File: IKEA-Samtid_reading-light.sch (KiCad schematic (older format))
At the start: 20 parts, among them IC1 ATTINY25-S, P1 CONN_2, U1 PT4115-SOT89-5

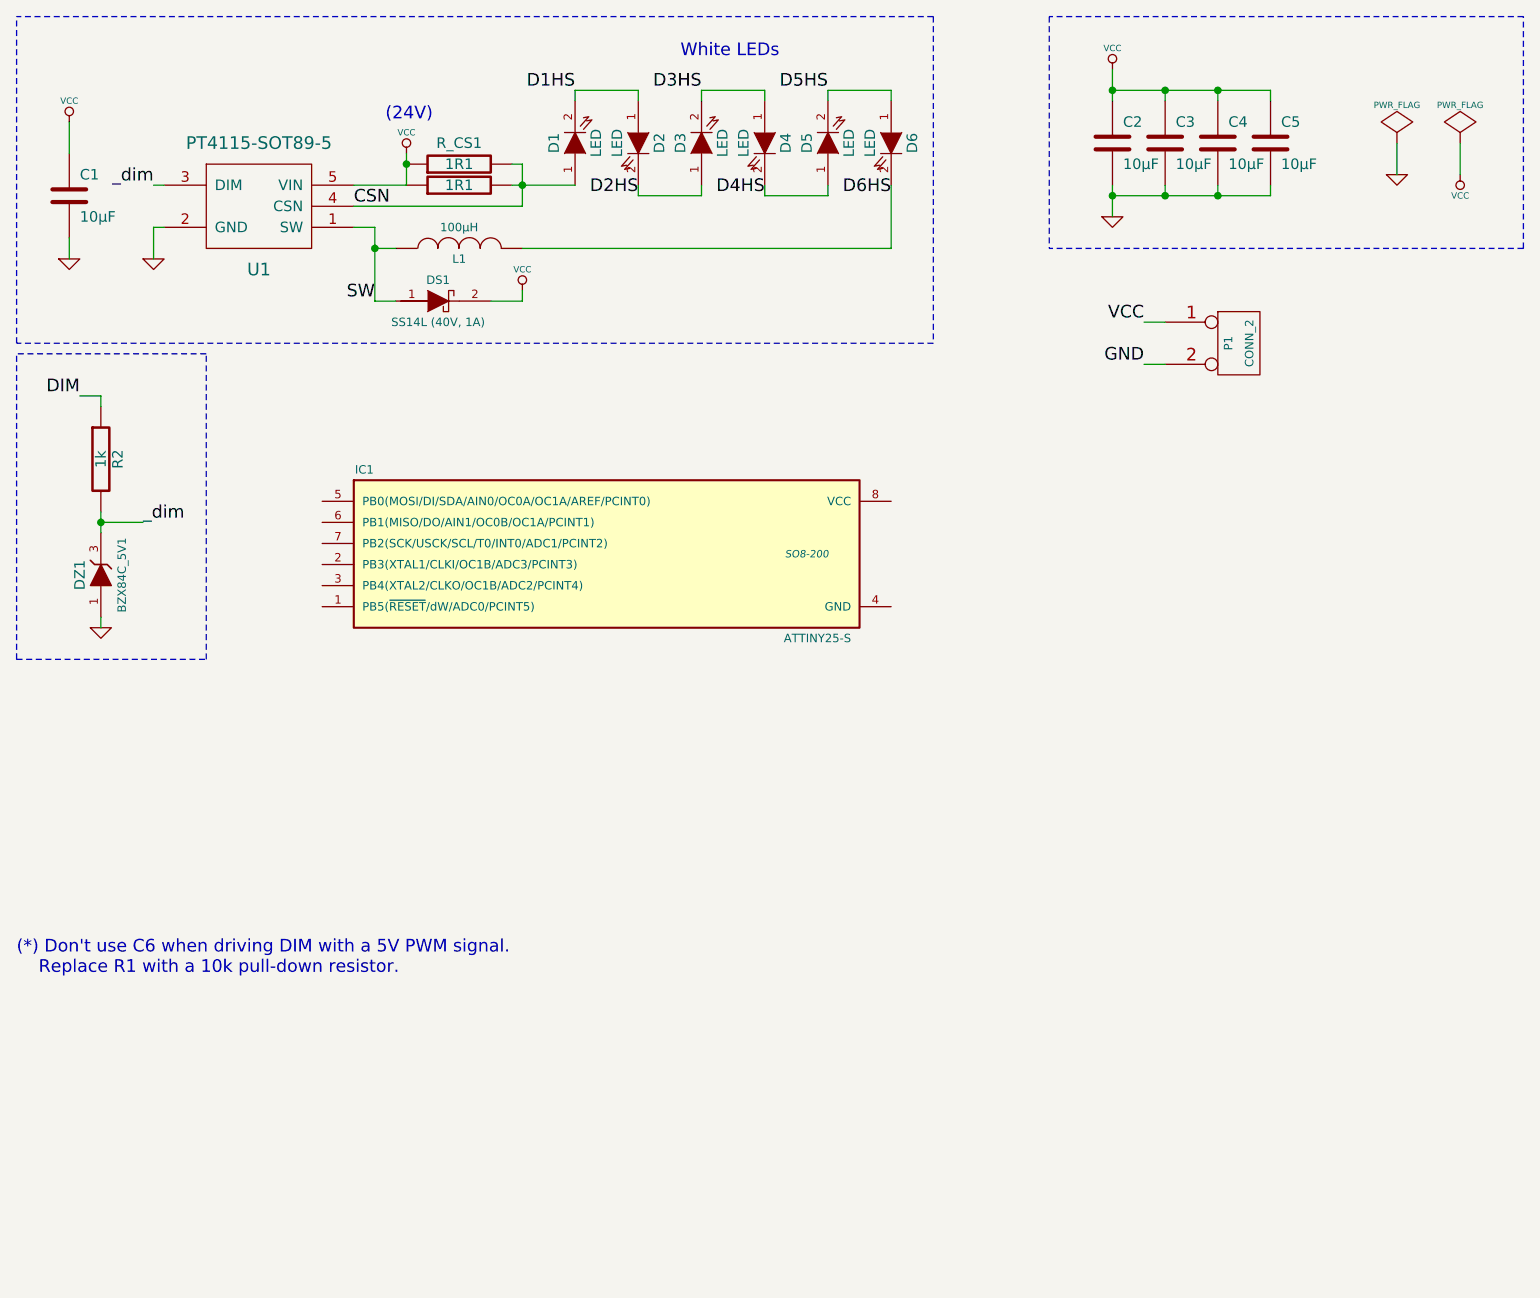
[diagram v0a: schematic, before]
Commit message: Shoving parts around.
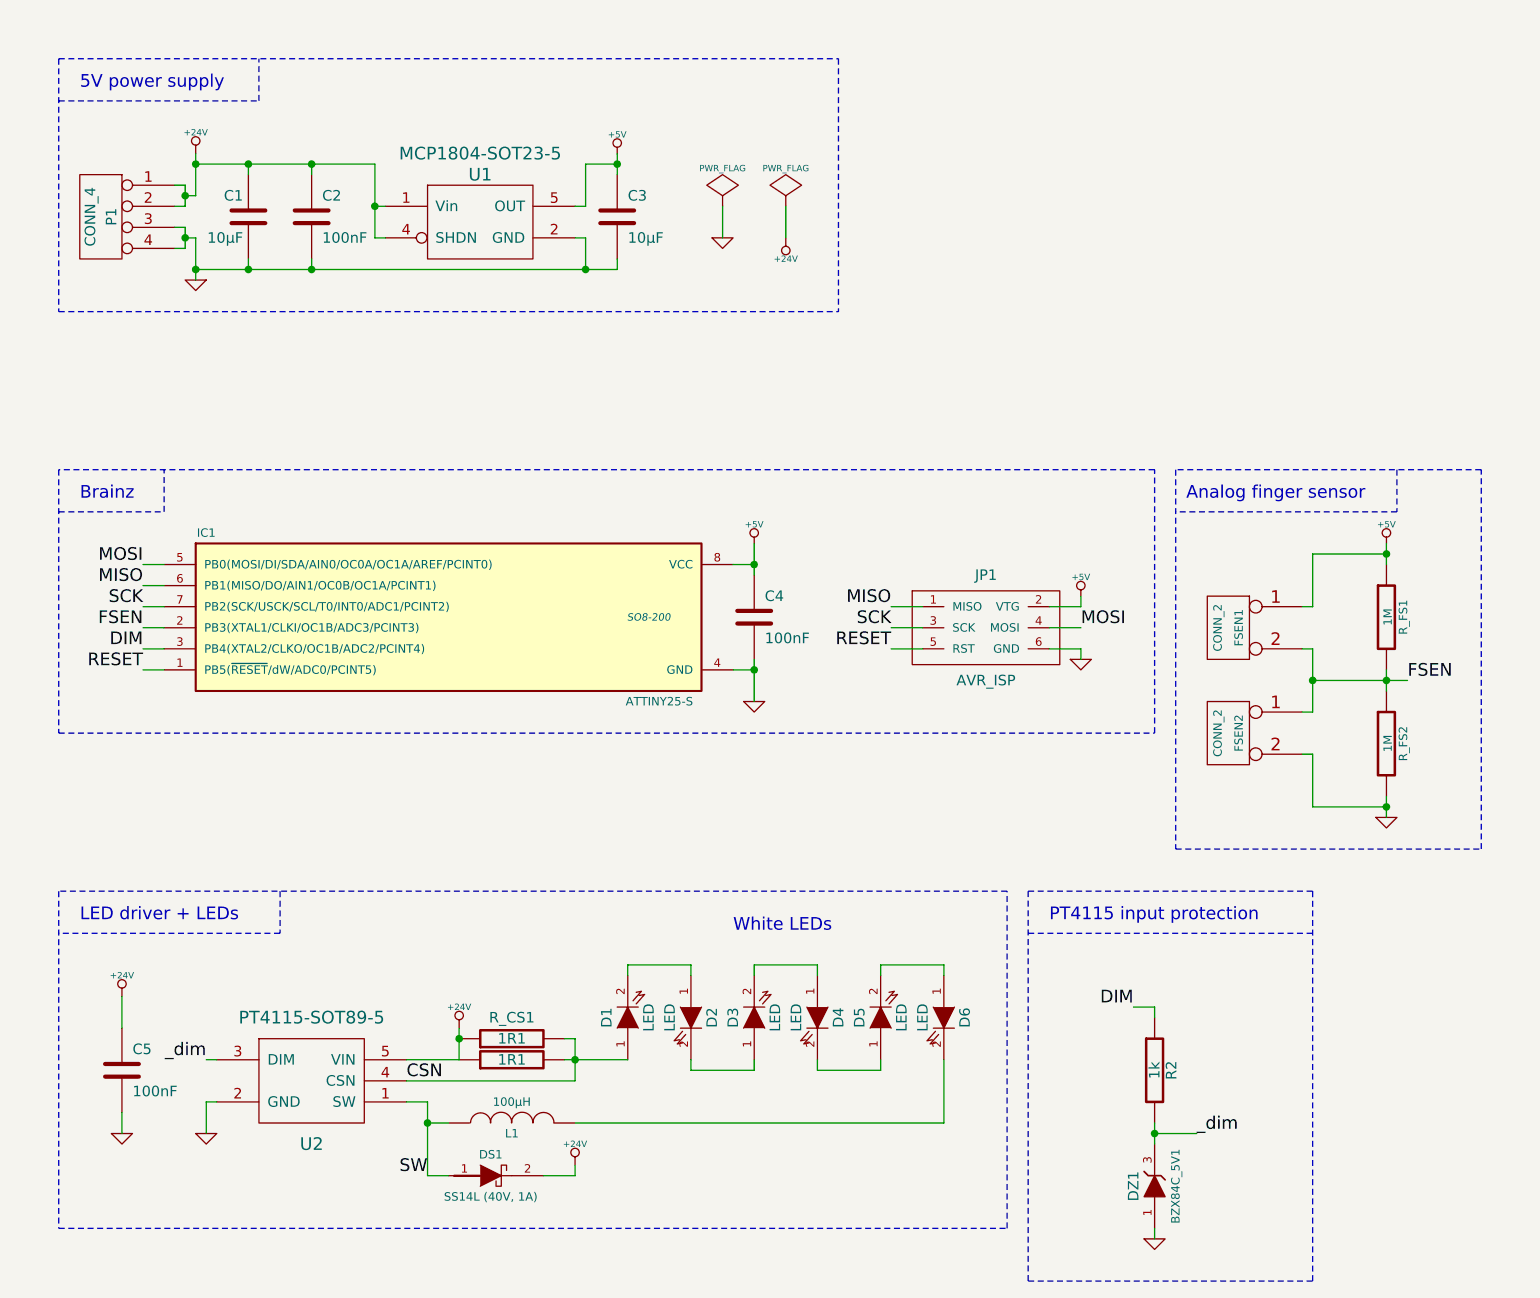
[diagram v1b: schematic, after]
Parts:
- removed C4: 10µF, symbol C
- removed P1: CONN_2, symbol CONN_2
- added C1: 10µF, symbol C
- added FSEN1, FSEN2: CONN_2, symbol CONN_2
- added JP1: AVR_ISP, symbol MADW__AVR_ISP
- added P1: CONN_4, symbol CONN_4
- added R_FS1, R_FS2: 1M, symbol R
- added U1: MCP1804-SOT23-5, symbol MADW__MCP1804-SOT23-5
- C2: value 10µF -> 100nF
- C4: renamed from C5; value 10µF -> 100nF
- C5: renamed from C1; value 10µF -> 100nF
- renumbered U1 to U2
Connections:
- net DIM: now also IC1.3 (PB4(XTAL2/CLKO/OC1B/ADC2/PCINT4))
- net GND: now also IC1.4 (GND), C1.2, FSEN2.2 (PM), JP1.6 (GND), P1.3 (P3), P1.4 (P4), R_FS2.2, U1.2 (GND)
- net RESET: now reaches IC1.1 (PB5(~RESET~/dW/ADC0/PCINT5))
- net RESET: now also JP1.5 (RST)
- net FSEN: now reaches IC1.2 (PB3(XTAL1/CLKI/OC1B/ADC3/PCINT3))
- net FSEN: now also FSEN1.2 (PM), FSEN2.1 (P1), R_FS1.2, R_FS2.1
- net MOSI: now reaches IC1.5 (PB0(MOSI/DI/SDA/AIN0/OC0A/OC1A/AREF/PCINT0))
- net MOSI: now also JP1.4 (MOSI)
- net MISO: now reaches IC1.6 (PB1(MISO/DO/AIN1/OC0B/OC1A/PCINT1))
- net MISO: now also JP1.1 (MISO)
- net SCK: now reaches IC1.7 (PB2(SCK/USCK/SCL/T0/INT0/ADC1/PCINT2))
- net SCK: now also JP1.3 (SCK)
- net +5V: now reaches IC1.8 (VCC)
- net +5V: now also C3.1, C4.1, FSEN1.1 (P1), JP1.2 (VTG), R_FS1.1, U1.5 (OUT)
- net D1HS: no longer names the net of D1.2 (K), D2.1 (A)
- net D2HS: no longer names the net of D2.2 (K), D3.1 (A)
- net D3HS: no longer names the net of D3.2 (K), D4.1 (A)
- net D4HS: no longer names the net of D4.2 (K), D5.1 (A)
- net D5HS: no longer names the net of D5.2 (K), D6.1 (A)
- net D6HS: no longer names the net of D6.2 (K), L1.2
- net VCC renamed +24V
- net +24V: now also C1.1, P1.1 (P1), P1.2 (P2), U1.1 (Vin), U1.4 (SHDN); no longer C3.1, C4.1
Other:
- note added: "5V power supply"
- note added: "Analog finger sensor"
- note added: "Brainz"
- note added: "LED driver + LEDs"
- note added: "PT4115 input protection"
- note removed: "(*) Don't use C6 when driving DIM with a 5V PWM signal.\n Replace R1 with a 10k pull-down resistor."
- note removed: "(24V)"
- moved on the sheet: C2, C4, C5, D1, D2, D3, D4, D5, D6, DS1, DZ1, IC1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
